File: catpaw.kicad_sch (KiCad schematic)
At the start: 26 parts, among them J1 m12,Acode,5pin,femalesocket, J3 Conn_01x01_Socket, J4 Conn_01x01_Socket, SW1 SW_DPST, U1 INA826, U2 ${SIM.PARAMS}

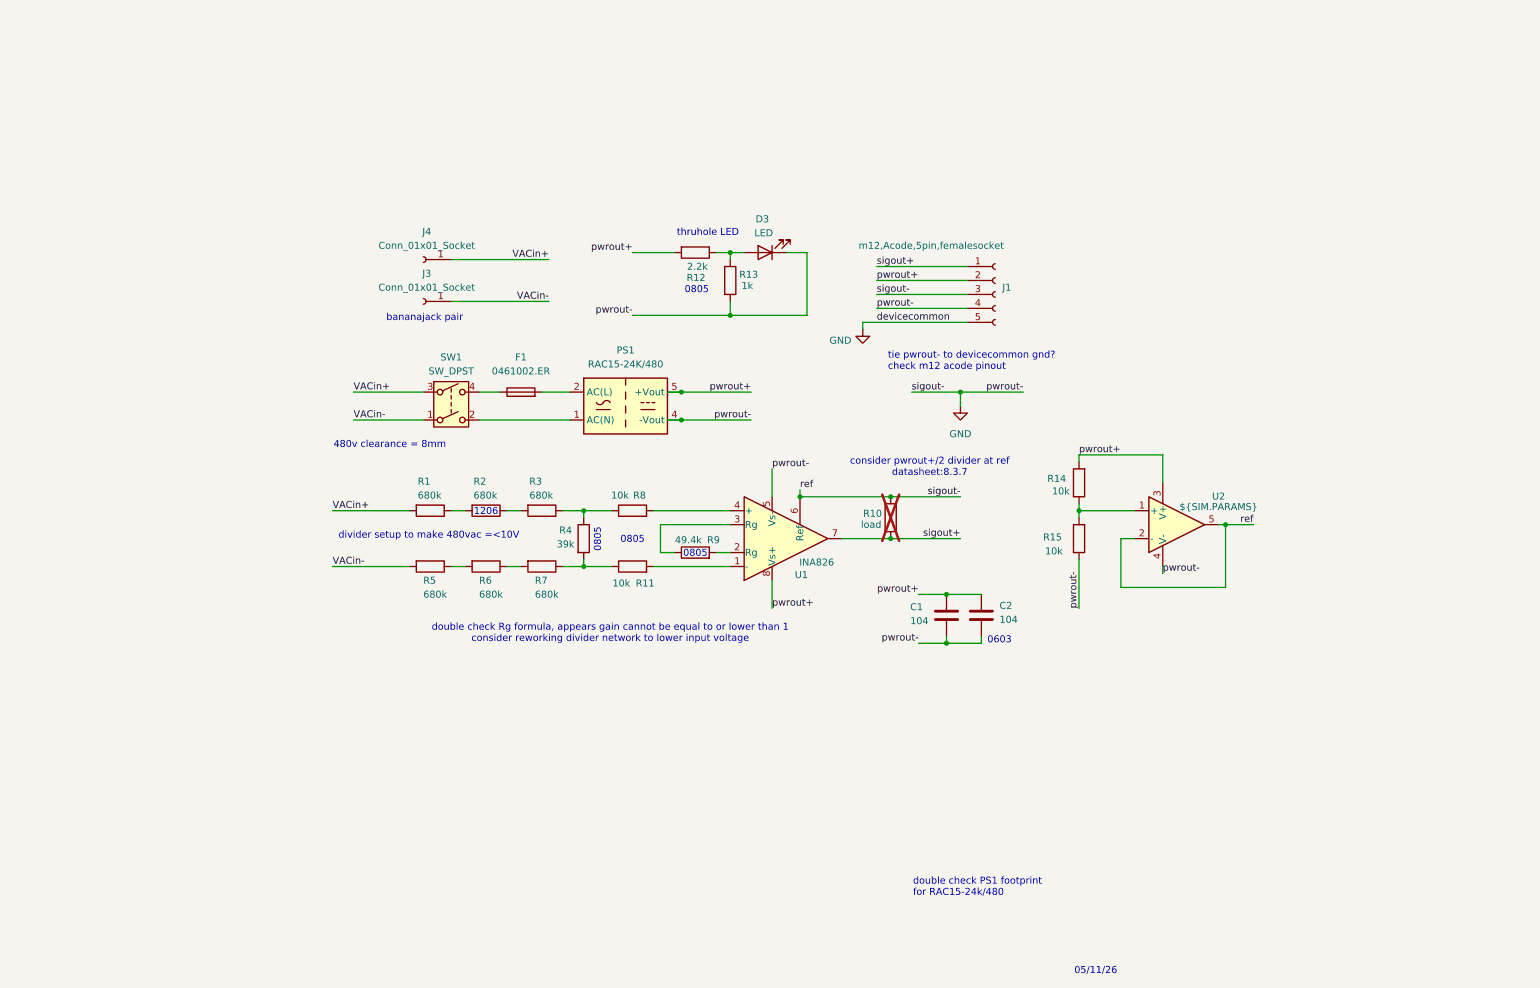
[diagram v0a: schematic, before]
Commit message: scheme rework
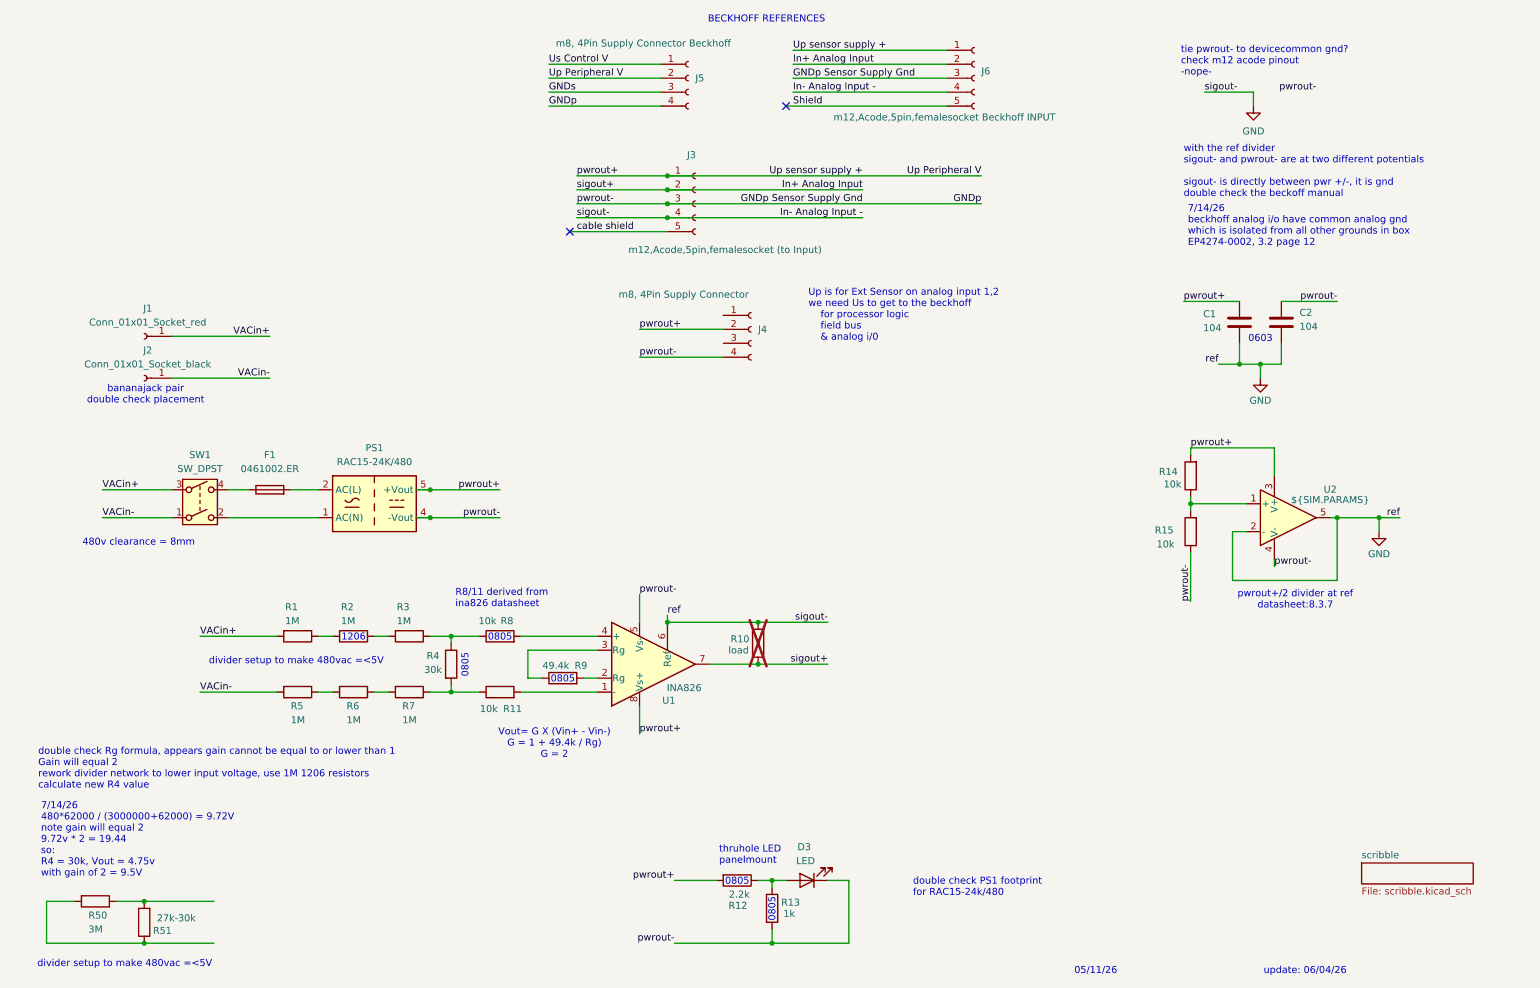
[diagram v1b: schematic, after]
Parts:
- added J4: m8, 4Pin Supply Connector, symbol Connector:Conn_01x04_Socket
- added J5: m8, 4Pin Supply Connector Beckhoff, symbol Connector:Conn_01x04_Socket
- added J6: m12,Acode,5pin,femalesocket Beckhoff INPUT, symbol Connector:Conn_01x05_Socket
- added R50: 3M, symbol Device:R
- added R51: 27k-30k, symbol Device:R
- J1: renamed from J4; value Conn_01x01_Socket -> Conn_01x01_Socket_red
- J2: renamed from J3; value Conn_01x01_Socket -> Conn_01x01_Socket_black
- J3: renamed from J1; value m12,Acode,5pin,femalesocket -> m12,Acode,5pin,femalesocket (to Input)
- R1, R2, R3, R5, R6, R7: value 680k -> 1M
- R4: value 39k -> 30k
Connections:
- net GND: now also J6.4 (Pin_4); no longer D3.1 (K), J3.3 (Pin_3), J3.5 (Pin_5), PS1.4 (-Vout), R13.2, R15.1, U1.5 (Vs-), U2.4 (V-)
- net pwrout+ renamed Up Peripheral V
- net Up Peripheral V: now also J3.1 (Pin_1), J4.2 (Pin_2), J5.2 (Pin_2), J6.1 (Pin_1); no longer C2.2, J3.2 (Pin_2)
- net sigout+ renamed In+ Analog Input
- net In+ Analog Input: now also J3.2 (Pin_2), J6.2 (Pin_2); no longer J3.1 (Pin_1)
- new net: R50.2, R51.1
- new net: R50.1, R51.2
- new net GNDp: C2.2, D3.1 (K), J3.3 (Pin_3), J4.4 (Pin_4), J5.4 (Pin_4), J6.3 (Pin_3), PS1.4 (-Vout), R13.2, R15.1, U1.5 (Vs-), U2.4 (V-)
- new net GNDs: J5.3 (Pin_3)
- new net Shield: J6.5 (Pin_5)
- new net Us Control V: J5.1 (Pin_1)
- new net cable shield: J3.5 (Pin_5)
- no-connect marks 0 -> 2
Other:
- added sheet scribble (scribble.kicad_sch)
- note added: "7/14/26 480*62000 / (3000000+62000) = 9.72V note gain will equal 2 9.72v * 2 = 19.44 so: R4 = 30k, Vout = 4.75v with gain of 2 = 9.5V"
- note added: "7/14/26 beckhoff analog i/o have common analog gnd which is isolated from all other grounds in box EP4274-0002, 3.2 page 12"
- note added: "BECKHOFF REFERENCES"
- note added: "R8/11 derived from ina826 datasheet"
- note added: "Up is for Ext Sensor on analog input 1,2 we need Us to get to the beckhoff for processor logic field bus & analog i/0"
- note added: "Vout= G X (Vin+ - Vin-) G = 1 + 49.4k / Rg) G = 2"
- note added: "bananajack pair double check placement"
- note added: "divider setup to make 480vac =<5V"
- note added: "double check Rg formula, appears gain cannot be equal to or lower than 1 Gain will equal 2 rework divider network to lower input voltage, use 1M 1206 resistors calculate new R4 value"
- note added: "pwrout+/2 divider at ref datasheet:8.3.7"
- note added: "thruhole LED panelmount"
- note added: "tie pwrout- to devicecommon gnd? check m12 acode pinout -nope-"
- note added: "update: 06/04/26"
- note added: "with the ref divider sigout- and pwrout- are at two different potentials sigout- is directly between pwr +/-, it is gnd double check the beckoff manual"
- note removed: "bananajack pair"
- note removed: "consider pwrout+/2 divider at ref datasheet:8.3.7"
- note removed: "divider setup to make 480vac =<10V"
- note removed: "double check Rg formula, appears gain cannot be equal to or lower than 1 consider reworking divider network to lower input voltage"
- note removed: "thruhole LED"
- note removed: "tie pwrout- to devicecommon gnd? check m12 acode pinout"
- moved on the sheet: C1, C2, D3, F1, J1, J2, J3, PS1, R1, R10, R11, R12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
